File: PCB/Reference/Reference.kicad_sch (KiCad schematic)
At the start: 27 parts, among them J1 Conn_01x04, U1 LMR16006XDDCR, U2 Barcode, U2 MD8942, U4 CH340X

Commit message: VCut
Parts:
- added V1, V2: ~, RevK:VCUT70, symbol RevK:VCUT
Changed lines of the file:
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@@
+    )
+  )
+  (symbol (lib_id "RevK:VCUT") (at 245.11 177.165 180) (unit 1)
+    (in_bom yes) (on_board yes) (dnp no) (fields_autoplaced)
+    (property "Reference" "V2" (at 245.11 178.435 0)
+      (effects (font (size 1.27 1.27)) hide)
+    )
+    (property "Value" "~" (at 245.11 177.165 0)
+      (effects (font (size 1.27 1.27)))
+    )
+    (property "Footprint" "RevK:VCUT70" (at 245.11 175.895 0)
+      (effects (font (size 1.27 1.27)) hide)
+    )
+    (property "Datasheet" "" (at 245.11 177.165 0)
+      (effects (font (size 1.27 1.27)) hide)
+    )
+    (instances
+      (project "Reference"
+        (path "/825c70b0-4860-42b7-97dc-86bfa46e06fd"
+          (reference "V2") (unit 1)
+        )
+      )
     )
   )
@@
         )
       )
+    )
+  )
+  (symbol (lib_id "RevK:VCUT") (at 245.11 170.815 0) (unit 1)
+    (in_bom yes) (on_board yes) (dnp no) (fields_autoplaced)
+    (property "Reference" "V1" (at 245.11 169.545 0)
+      (effects (font (size 1.27 1.27)) hide)
+    )
+    (property "Value" "~" (at 245.11 170.815 0)
+      (effects (font (size 1.27 1.27)))
+    )
+    (property "Footprint" "RevK:VCUT70" (at 245.11 172.085 0)
+      (effects (font (size 1.27 1.27)) hide)
+    )
+    (property "Datasheet" "" (at 245.11 170.815 0)
+      (effects (font (size 1.27 1.27)) hide)
+    )
+    (instances
+      (project "Reference"
+        (path "/825c70b0-4860-42b7-97dc-86bfa46e06fd"
+          (reference "V1") (unit 1)
+        )
+      )

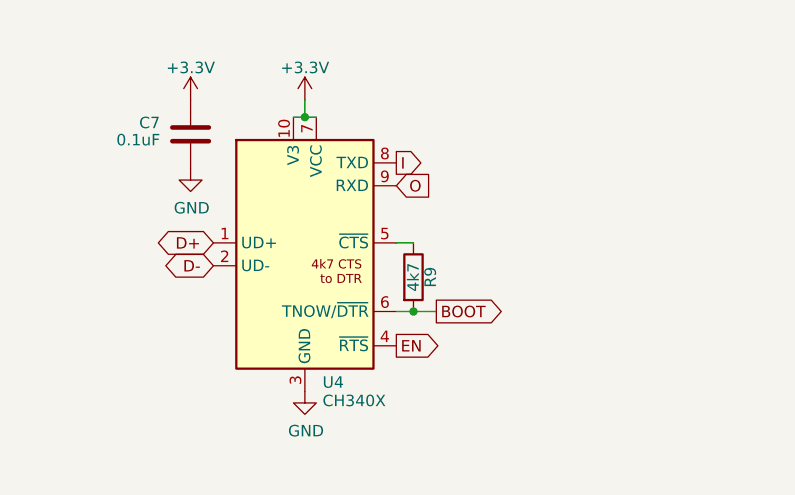
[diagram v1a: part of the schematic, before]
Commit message: CH340X DTR
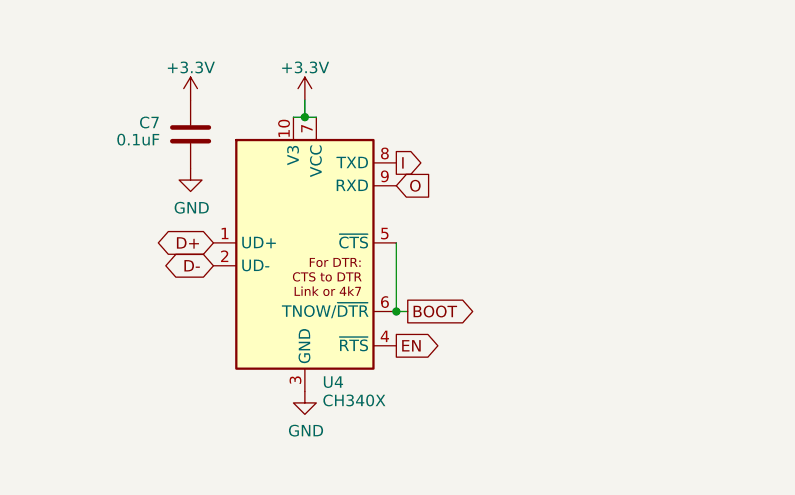
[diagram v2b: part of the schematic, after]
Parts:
- removed R9: 4k7, RevK:R_0402, symbol Device:R
- V1, V2: now left out of the parts list
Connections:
- net BOOT: now also U4.5 (~{CTS})
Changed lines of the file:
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@@
   (junction (at 93.345 52.07) (diameter 0) (color 0 0 0 0)
   )
-  (junction (at 120.015 160.02) (diameter 0) (color 0 0 0 0)
-  )
   (junction (at 107.95 138.43) (diameter 0) (color 0 0 0 0)
   )
   (junction (at 93.345 49.53) (diameter 0) (color 0 0 0 0)
+  )
+  (junction (at 118.11 160.02) (diameter 0) (color 0 0 0 0)
   )
   (junction (at 97.155 57.15) (diameter 0) (color 0 0 0 0)
@@
     (stroke (width 0) (type default))
   )
+  (wire (pts (xy 118.11 152.4) (xy 118.11 160.02))
+    (stroke (width 0) (type default))
+  )
   (wire (pts (xy 97.155 62.865) (xy 94.615 62.865))
     (stroke (width 0) (type default))
@@
     (stroke (width 0) (type default))
   )
-  (wire (pts (xy 122.555 160.02) (xy 120.015 160.02))
-    (stroke (width 0) (type default))
-  )
-  (wire (pts (xy 120.015 152.4) (xy 118.11 152.4))
+  (wire (pts (xy 118.11 160.02) (xy 119.38 160.02))
     (stroke (width 0) (type default))
   )
   (wire (pts (xy 97.155 57.15) (xy 104.775 57.15))
-    (stroke (width 0) (type default))
-  )
-  (wire (pts (xy 120.015 160.02) (xy 118.11 160.02))
     (stroke (width 0) (type default))
   )
@@
     )
   )
-  (global_label "BOOT" (shape output) (at 122.555 160.02 0) (fields_autoplaced)
+  (global_label "BOOT" (shape output) (at 119.38 160.02 0) (fields_autoplaced)
     (effects (font (size 1.27 1.27)) (justify left))
-    (property "Intersheetrefs" "${INTERSHEET_REFS}" (at 129.7052 160.02 0)
+    (property "Intersheetrefs" "${INTERSHEET_REFS}" (at 126.5302 160.02 0)
       (effects (font (size 1.27 1.27)) (justify left) hide)
     )
@@
   )
   (symbol (lib_id "RevK:VCUT") (at 245.11 177.165 180) (unit 1)
-    (in_bom yes) (on_board yes) (dnp no) (fields_autoplaced)
+    (in_bom no) (on_board yes) (dnp no) (fields_autoplaced)
     (property "Reference" "V2" (at 245.11 178.435 0)
       (effects (font (size 1.27 1.27)) hide)
@@
     )
     (property "Datasheet" "" (at 245.11 177.165 0)
+      (effects (font (size 1.27 1.27)) hide)
+    )
+    (property "Sim.Enable" "0" (at 245.11 177.165 0)
       (effects (font (size 1.27 1.27)) hide)
     )
@@
     )
   )
-  (symbol (lib_id "Device:R") (at 120.015 156.21 0) (unit 1)
-    (in_bom yes) (on_board yes) (dnp no)
-    (property "Reference" "R9" (at 121.92 156.21 90)
-      (effects (font (size 1.27 1.27)))
-    )
-    (property "Value" "4k7" (at 120.015 156.21 90)
-      (effects (font (size 1.27 1.27)))
-    )
-    (property "Footprint" "RevK:R_0402" (at 118.237 156.21 90)
-      (effects (font (size 1.27 1.27)) hide)
-    )
-    (property "Datasheet" "~" (at 120.015 156.21 0)
-      (effects (font (size 1.27 1.27)) hide)
-    )
-    (pin "1")
-    (pin "2")
-    (instances
-      (project "Reference"
-        (path "/825c70b0-4860-42b7-97dc-86bfa46e06fd"
-          (reference "R9") (unit 1)
-        )
-      )
-      (project "Generic"
-        (path "/babeabf2-f3b0-4ed5-8d9e-0215947e6cf3"
-          (reference "R6") (unit 1)
-        )
-      )
-    )
-  )
   (symbol (lib_id "Device:R") (at 100.965 62.865 90) (unit 1)
     (in_bom yes) (on_board yes) (dnp no)
@@
   )
   (symbol (lib_id "RevK:VCUT") (at 245.11 170.815 0) (unit 1)
-    (in_bom yes) (on_board yes) (dnp no) (fields_autoplaced)
+    (in_bom no) (on_board yes) (dnp no) (fields_autoplaced)
     (property "Reference" "V1" (at 245.11 169.545 0)
       (effects (font (size 1.27 1.27)) hide)
@@
       (effects (font (size 1.27 1.27)) hide)
     )
+    (property "Sim.Enable" "0" (at 245.11 170.815 0)
+      (effects (font (size 1.27 1.27)) hide)
+    )
